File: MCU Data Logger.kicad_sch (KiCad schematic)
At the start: 25 parts, among them U1 24LC1025, U2 24LC1025, U3 ATmega328P, U4 DS1337S_, Y1 16MHz, Y2 32.768 KHz

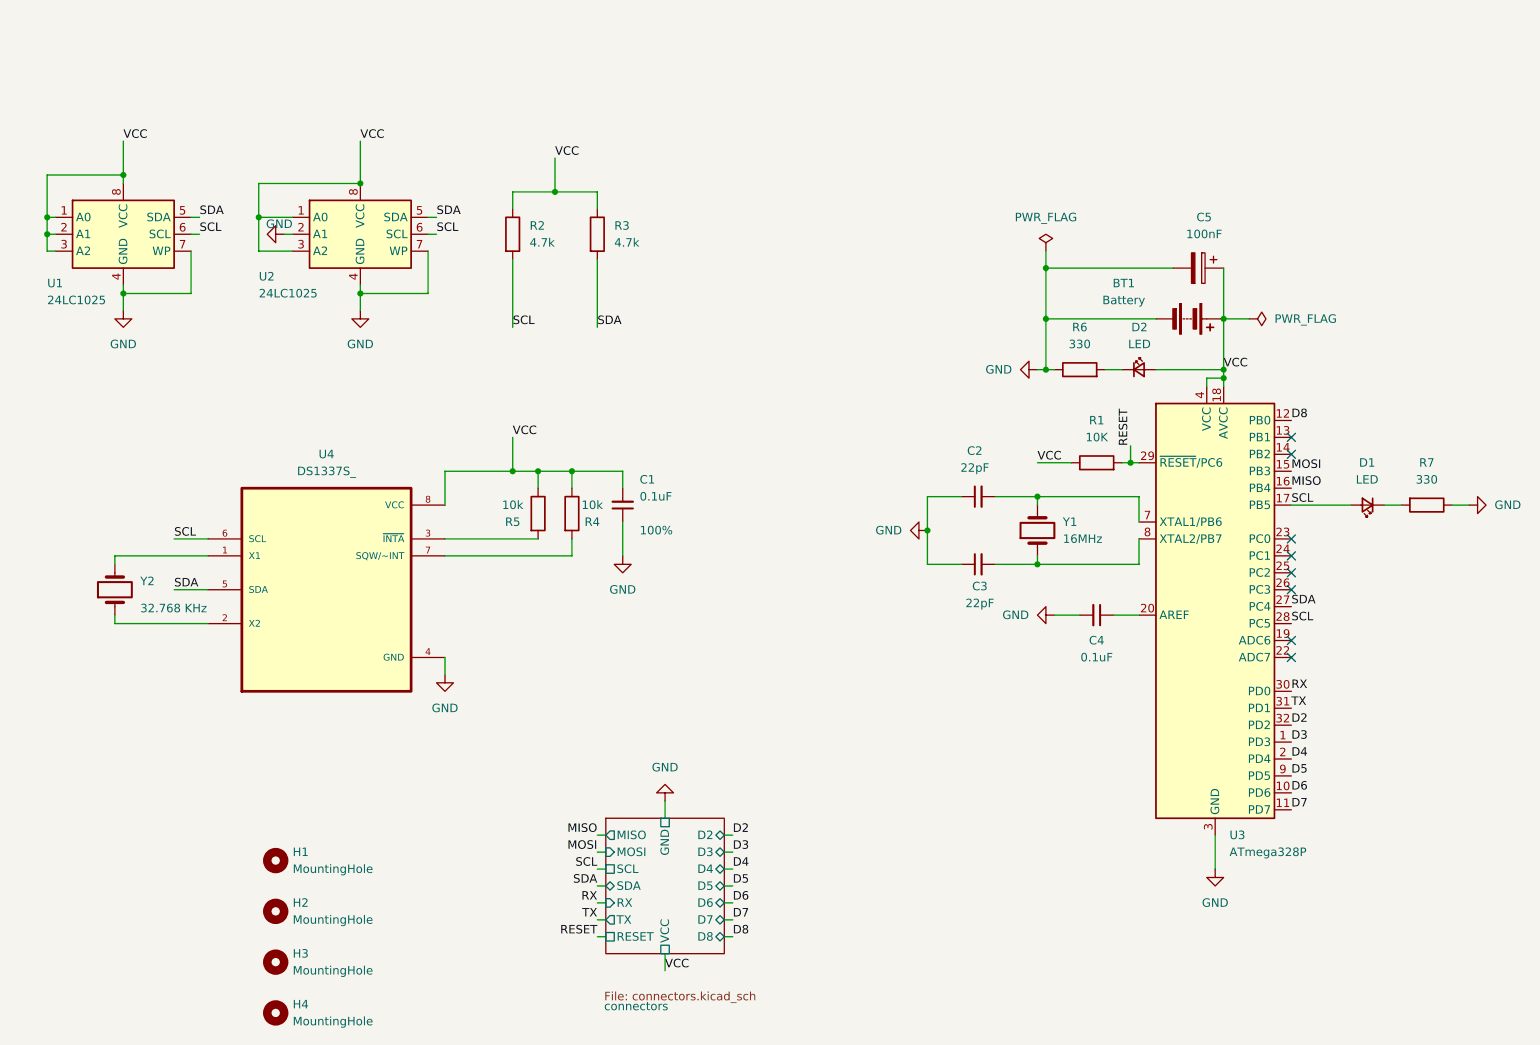
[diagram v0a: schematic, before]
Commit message: Finishing Schematic
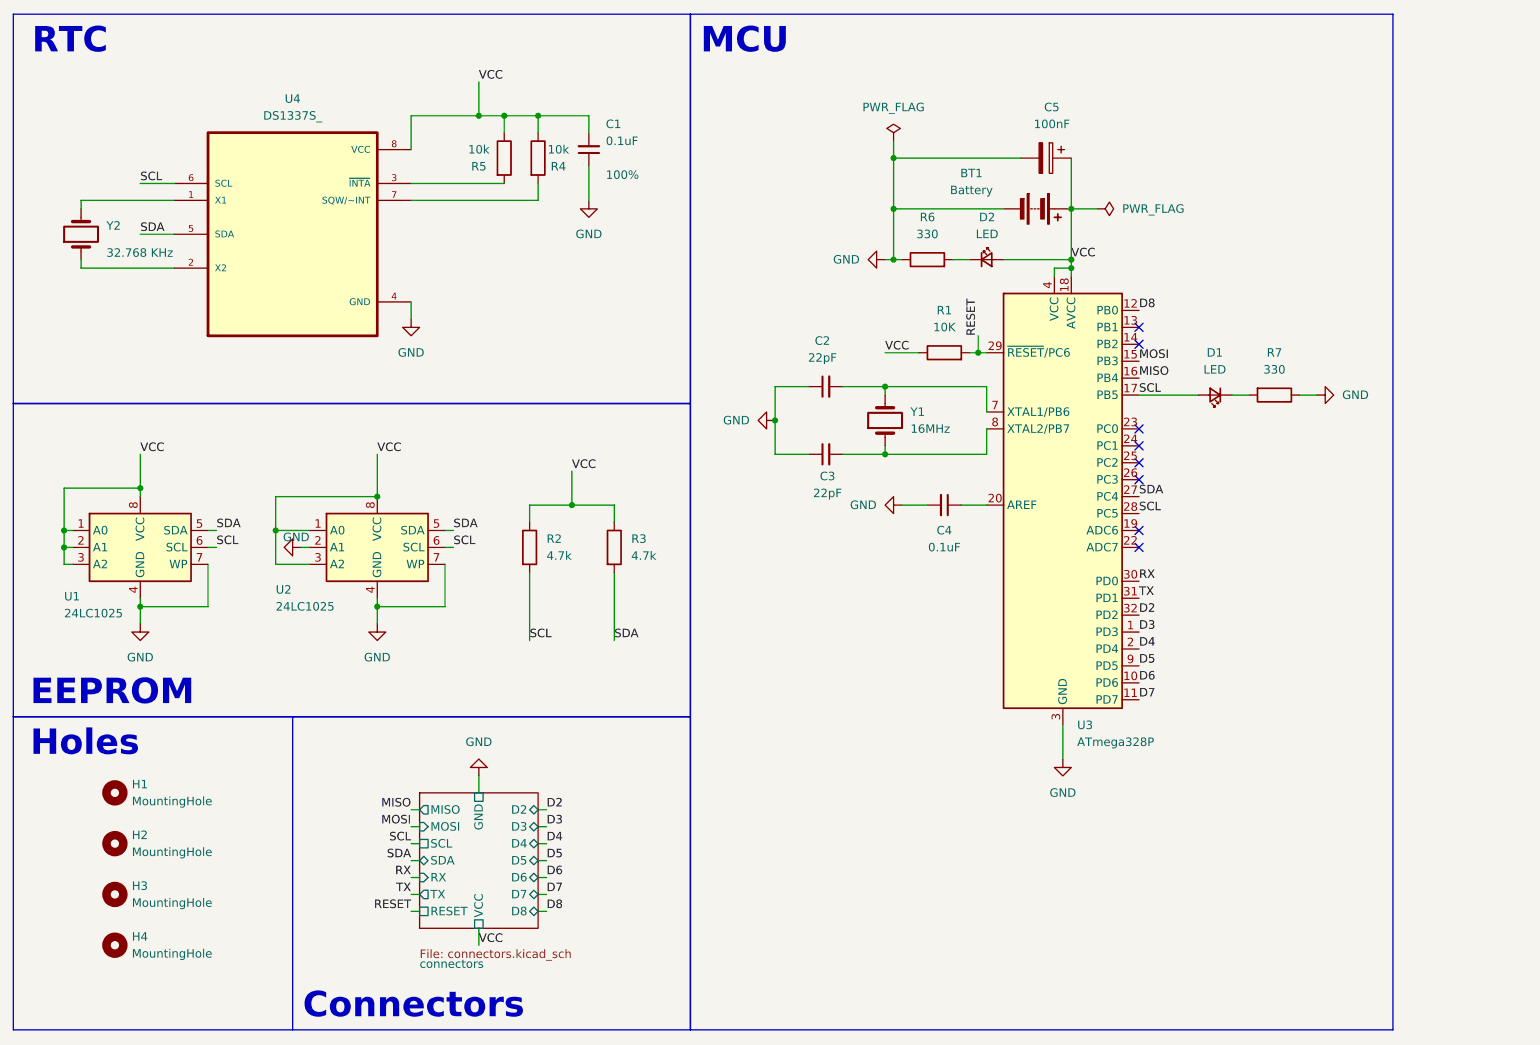
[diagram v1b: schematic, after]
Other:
- note added: "Connectors"
- note added: "EEPROM"
- note added: "Holes"
- note added: "MCU"
- note added: "RTC"
- moved on the sheet: BT1, C1, C2, C3, C4, C5, D1, D2, H1, H2, H3, H4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
